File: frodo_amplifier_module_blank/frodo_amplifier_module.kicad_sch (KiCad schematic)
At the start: 19 parts, among them IC1 INA826AID, IC2 AS321KTR-G1, J1 Conn_01x01_Socket, J2 Conn_01x01_Socket, J3 Conn_01x01_Socket, J4 Conn_01x01_Socket, J5 Conn_01x01_Socket, J6 Conn_01x01_Socket, J7 Conn_01x01_Socket, J8 Conn_01x01_Socket

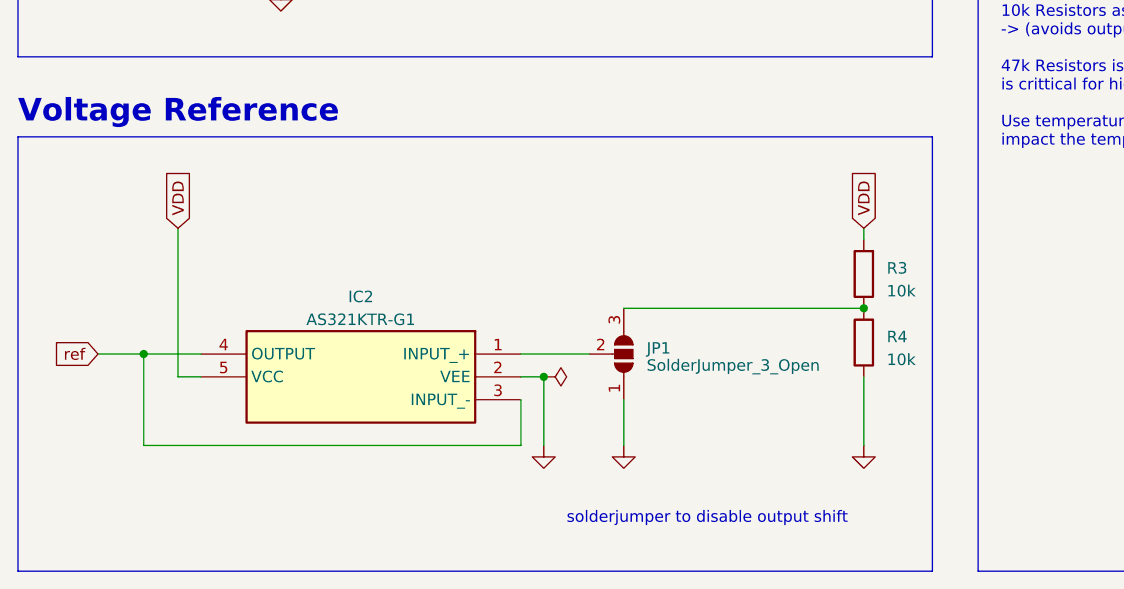
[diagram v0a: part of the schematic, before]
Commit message: fixed my messup
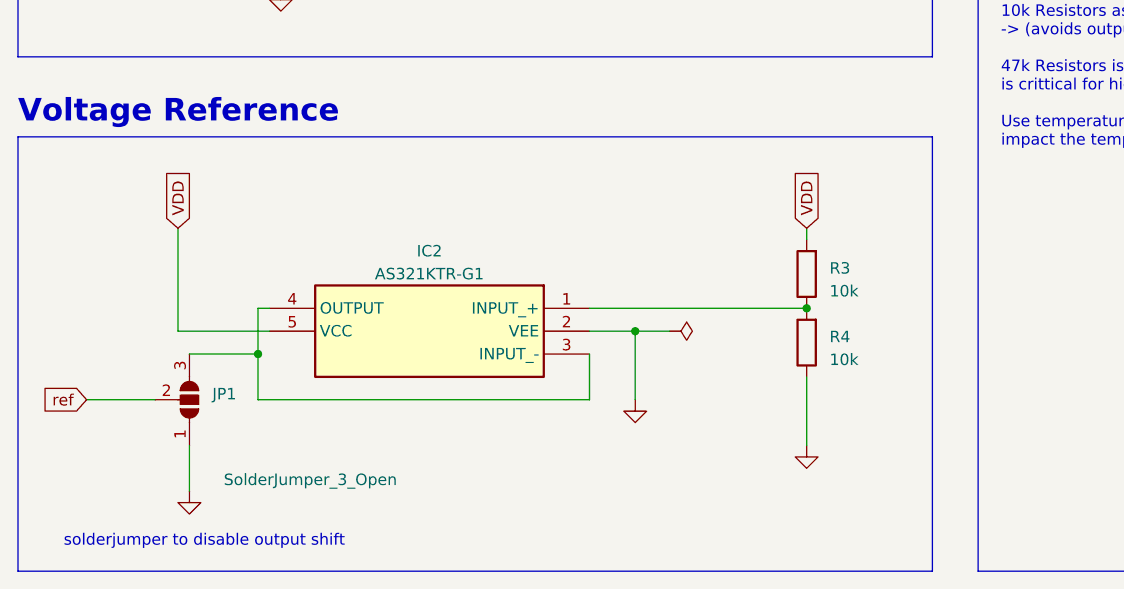
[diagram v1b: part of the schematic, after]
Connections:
- net ref: now also JP1.2 (C); no longer IC2.3 (INPUT_-), IC2.4 (OUTPUT)
- net at IC2.1 (INPUT_+): now also R3.1, R4.2; no longer JP1.2 (C)
- new net: IC2.3 (INPUT_-), IC2.4 (OUTPUT), JP1.3 (B)
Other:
- moved on the sheet: IC2, R3, R4

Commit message: updated mounting holes and footprints of c2 and fb1
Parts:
- C2: footprint Capacitor_SMD:C_0402_1005Metric_Pad0.74x0.62mm_HandSolder -> Capacitor_SMD:C_0603_1608Metric
- FB1: footprint Inductor_SMD:L_0402_1005Metric_Pad0.77x0.64mm_HandSolder -> Inductor_SMD:L_0603_1608Metric
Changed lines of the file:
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@@
       (effects (font (size 1.27 1.27)) (justify left))
     )
-    (property "Footprint" "Capacitor_SMD:C_0402_1005Metric_Pad0.74x0.62mm_HandSolder" (at 83.5152 55.88 0)
+    (property "Footprint" "Capacitor_SMD:C_0603_1608Metric" (at 83.5152 55.88 0)
       (effects (font (size 1.27 1.27)) hide)
     )
@@
       (effects (font (size 1.27 1.27)))
     )
-    (property "Footprint" "Inductor_SMD:L_0402_1005Metric_Pad0.77x0.64mm_HandSolder" (at 66.04 44.958 90)
-      (effects (font (size 1.27 1.27)) hide)
-    )
+    (property "Footprint" "Inductor_SMD:L_0603_1608Metric" (at 66.04 44.958 90)
+      (effects (font (size 1.27 1.27)) hide)
+    )
